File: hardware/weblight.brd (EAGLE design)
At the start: 43.2 x 12.7 mm, 16 parts, among them U1 ATtiny85-20SU

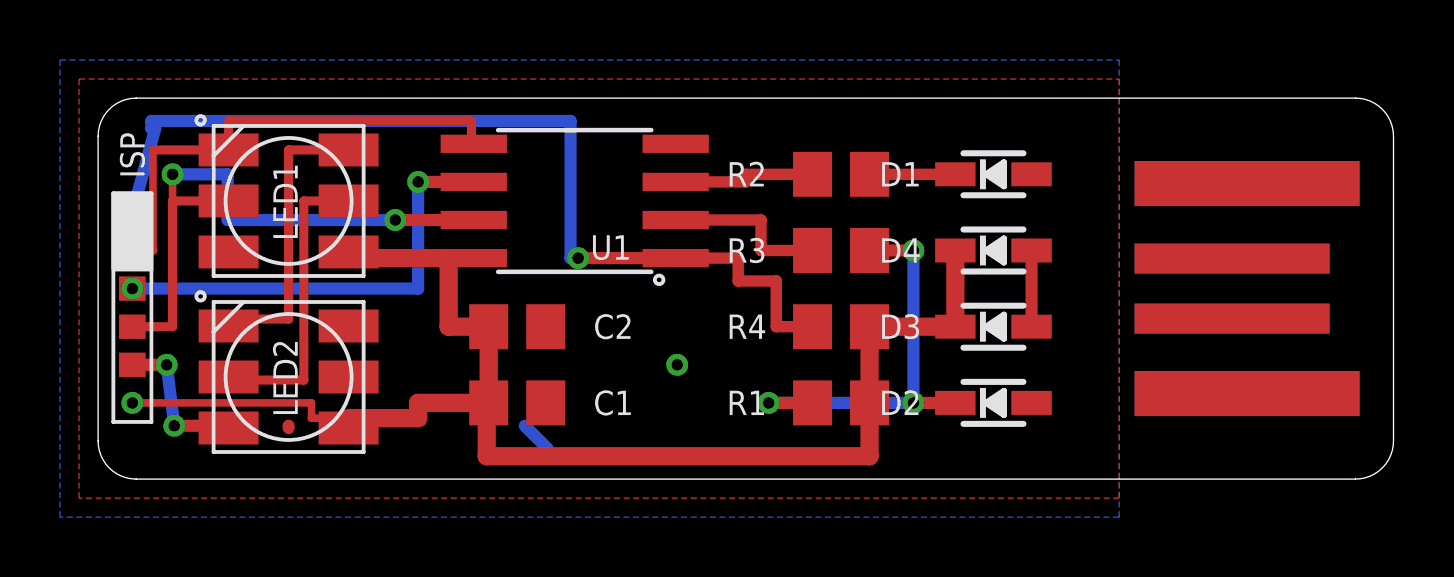
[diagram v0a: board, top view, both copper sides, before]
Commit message: Checkpoint #3, some connectors
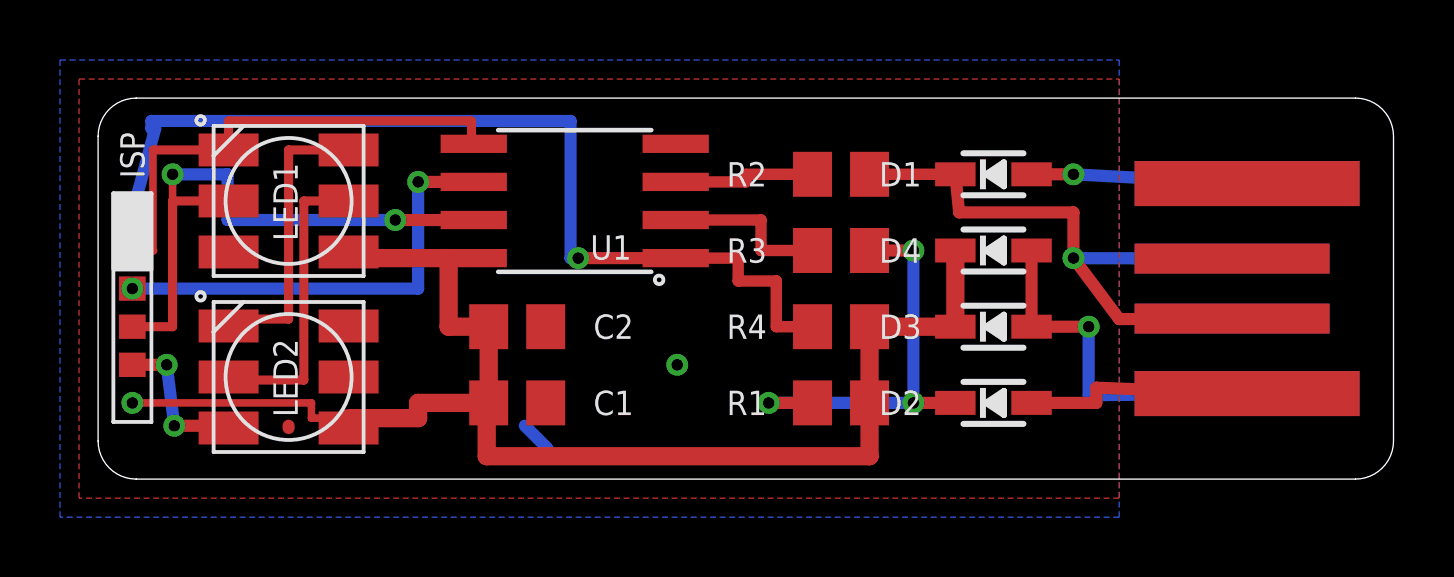
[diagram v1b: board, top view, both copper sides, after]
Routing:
- net USB_D_PLUS_RAW: track 2.86 -> 21.1 mm, vias 0 -> 1
- net GND: track 6.23 -> 21.1 mm, vias 3 -> 4
- net 5V: track 2.54 -> 12.0 mm, vias 0 -> 1
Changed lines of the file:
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@@
 <via x="2.286" y="3.81" extent="1-16" drill="0.381"/>
 <wire x1="2.286" y1="3.81" x2="2.54" y2="1.778" width="0.4064" layer="16"/>
+<wire x1="31.115" y1="10.16" x2="32.512" y2="10.16" width="0.4064" layer="1"/>
+<via x="32.512" y="10.16" extent="1-16" drill="0.381"/>
+<wire x1="32.512" y1="10.16" x2="38.3" y2="9.85" width="0.4064" layer="16"/>
+<wire x1="31.115" y1="2.54" x2="33.274" y2="2.54" width="0.4064" layer="1"/>
+<wire x1="33.274" y1="2.54" x2="33.274" y2="3.048" width="0.4064" layer="1"/>
+<wire x1="33.274" y1="3.048" x2="38.3" y2="2.85" width="0.4064" layer="1"/>
 <wire x1="38.3" y1="2.85" x2="38.3" y2="9.85" width="0" layer="19" extent="1-16"/>
-<wire x1="31.115" y1="10.16" x2="38.3" y2="9.85" width="0" layer="19" extent="1-16"/>
 </signal>
 <signal name="USB_D_MINUS">
@@
 <contactref element="J-BOT" pad="USB_P"/>
 <wire x1="28.575" y1="10.16" x2="25.715" y2="10.16" width="0.381" layer="1"/>
-<wire x1="37.8" y1="7.35" x2="37.8" y2="5.35" width="0" layer="19" extent="1-16"/>
-<wire x1="28.575" y1="10.16" x2="37.8" y2="7.35" width="0" layer="19" extent="1-16"/>
+<wire x1="37.8" y1="7.35" x2="32.512" y2="7.366" width="0.4064" layer="16"/>
+<via x="32.512" y="7.366" extent="1-16" drill="0.381"/>
+<wire x1="32.512" y1="7.366" x2="34.036" y2="5.334" width="0.4064" layer="1"/>
+<wire x1="34.036" y1="5.334" x2="37.8" y2="5.35" width="0.4064" layer="1"/>
+<wire x1="32.512" y1="7.366" x2="32.512" y2="8.89" width="0.4064" layer="1"/>
+<wire x1="32.512" y1="8.89" x2="28.702" y2="8.89" width="0.4064" layer="1"/>
+<wire x1="28.702" y1="8.89" x2="28.575" y2="10.16" width="0.4064" layer="1"/>
 </signal>
 <signal name="USB_D_PLUS">
@@
 <contactref element="D4" pad="A"/>
 <wire x1="31.115" y1="7.62" x2="31.115" y2="5.08" width="0.4064" layer="1"/>
+<wire x1="38.3" y1="2.85" x2="33.02" y2="2.794" width="0.4064" layer="16"/>
+<wire x1="33.02" y1="2.794" x2="33.02" y2="5.08" width="0.4064" layer="16"/>
+<via x="33.02" y="5.08" extent="1-16" drill="0.381"/>
+<wire x1="33.02" y1="5.08" x2="31.115" y2="5.08" width="0.4064" layer="1"/>
 <wire x1="38.3" y1="2.85" x2="38.3" y2="9.85" width="0" layer="19" extent="1-16"/>
-<wire x1="31.115" y1="7.62" x2="38.3" y2="9.85" width="0" layer="19" extent="1-1"/>
 </signal>
 </signals>
